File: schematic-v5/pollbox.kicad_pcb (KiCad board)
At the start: 2 copper layers, 50.8 x 74.9 mm, 24 parts, among them P1 CONN_01X15, P10 CONN_01X04, P2 CONN_02X03, P20 CONN_01X04, P3 CONN_01X15, P30 CONN_01X04, P40 CONN_01X04, P50 CONN_01X04, U1 NodeMCU_1.0, U2 ULN2803

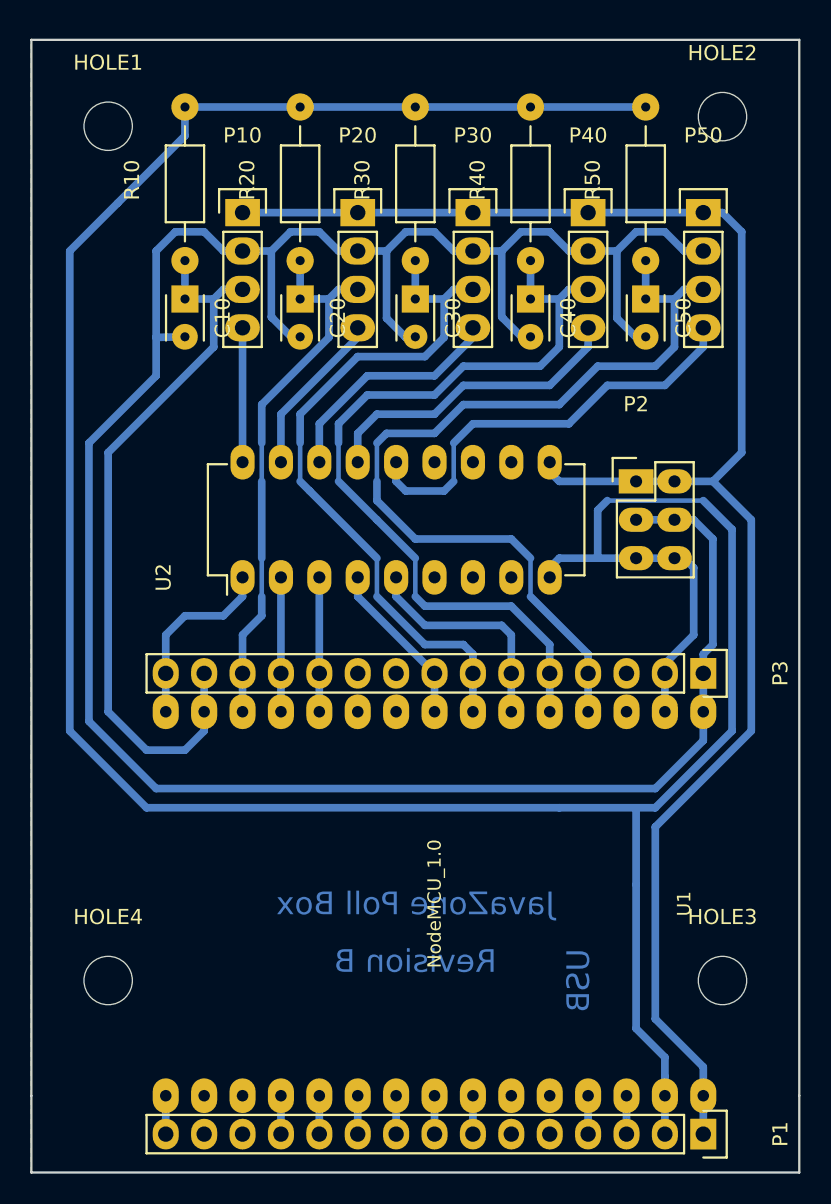
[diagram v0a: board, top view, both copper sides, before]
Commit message: some more routes cleanup
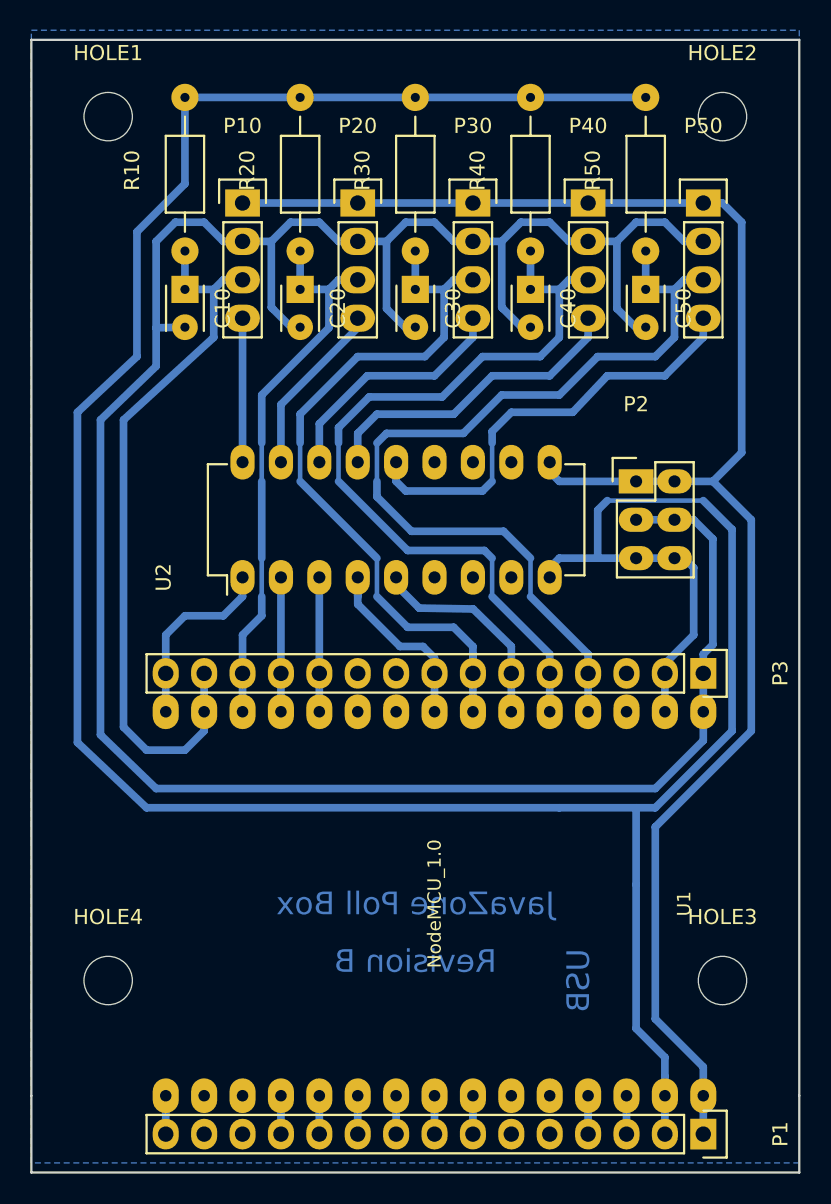
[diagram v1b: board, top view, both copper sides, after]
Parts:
- moved P10 0.64 mm to (91.4, 55.2)
- moved P20 0.64 mm to (99.1, 55.2)
- moved P30 0.64 mm to (106.7, 55.2)
- moved P40 0.64 mm to (114.3, 55.2)
- moved P50 0.64 mm to (121.9, 55.2)
- moved C10 0.63 mm to (87.6, 61.0)
- moved C20 0.63 mm to (95.2, 61.0)
- moved C30 0.63 mm to (102.9, 61.0)
- moved C40 0.63 mm to (110.5, 61.0)
- moved C50 0.63 mm to (118.1, 61.0)
- moved HOLE1 0.63 mm to (82.5, 49.5)
- moved R10 0.63 mm to (87.6, 53.3)
- moved R20 0.63 mm to (95.2, 53.3)
- moved R30 0.63 mm to (102.9, 53.3)
- moved R40 0.63 mm to (110.5, 53.3)
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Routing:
- net /SWITCH_3: track 47.1 -> 49.3 mm
- net /LED_4: track 11.0 -> 13.2 mm
- net /LED_2_OUT: track 11.0 -> 12.3 mm
- net /LED_3_OUT: track 16.3 -> 17.6 mm
- net /LED_5: track 15.0 -> 14.1 mm
- net /LED_5_OUT: track 29.2 -> 29.9 mm
- net /SWITCH_2: track 36.3 -> 36.9 mm
- net +5V: track 111.4 -> 112.0 mm
